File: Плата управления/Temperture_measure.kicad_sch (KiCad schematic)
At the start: 5 parts, among them U8 LMV321

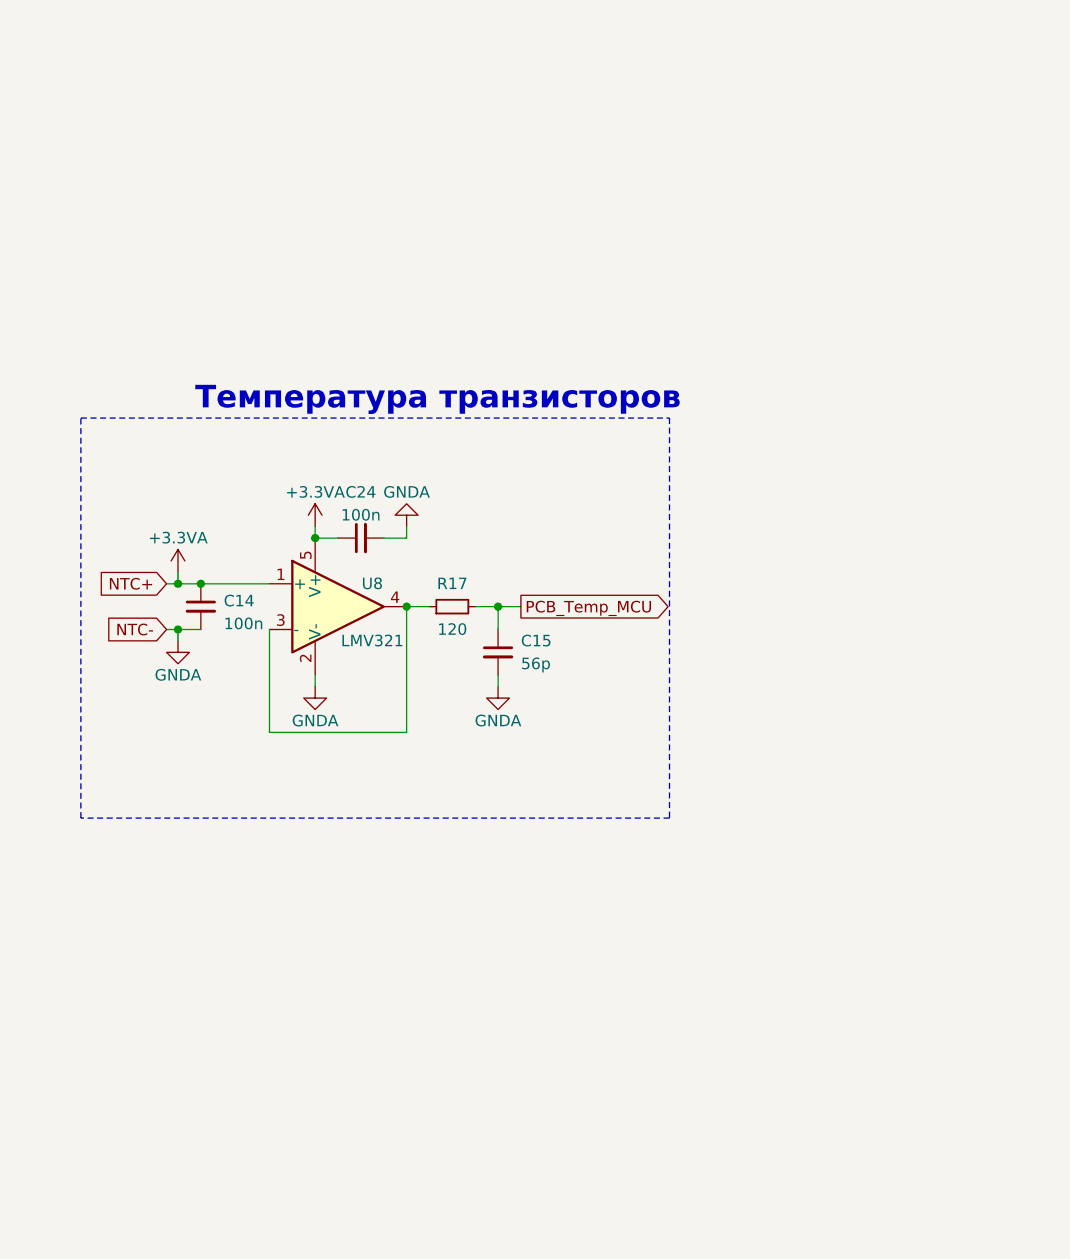
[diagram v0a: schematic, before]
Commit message: Новые драйвера и разъёмы
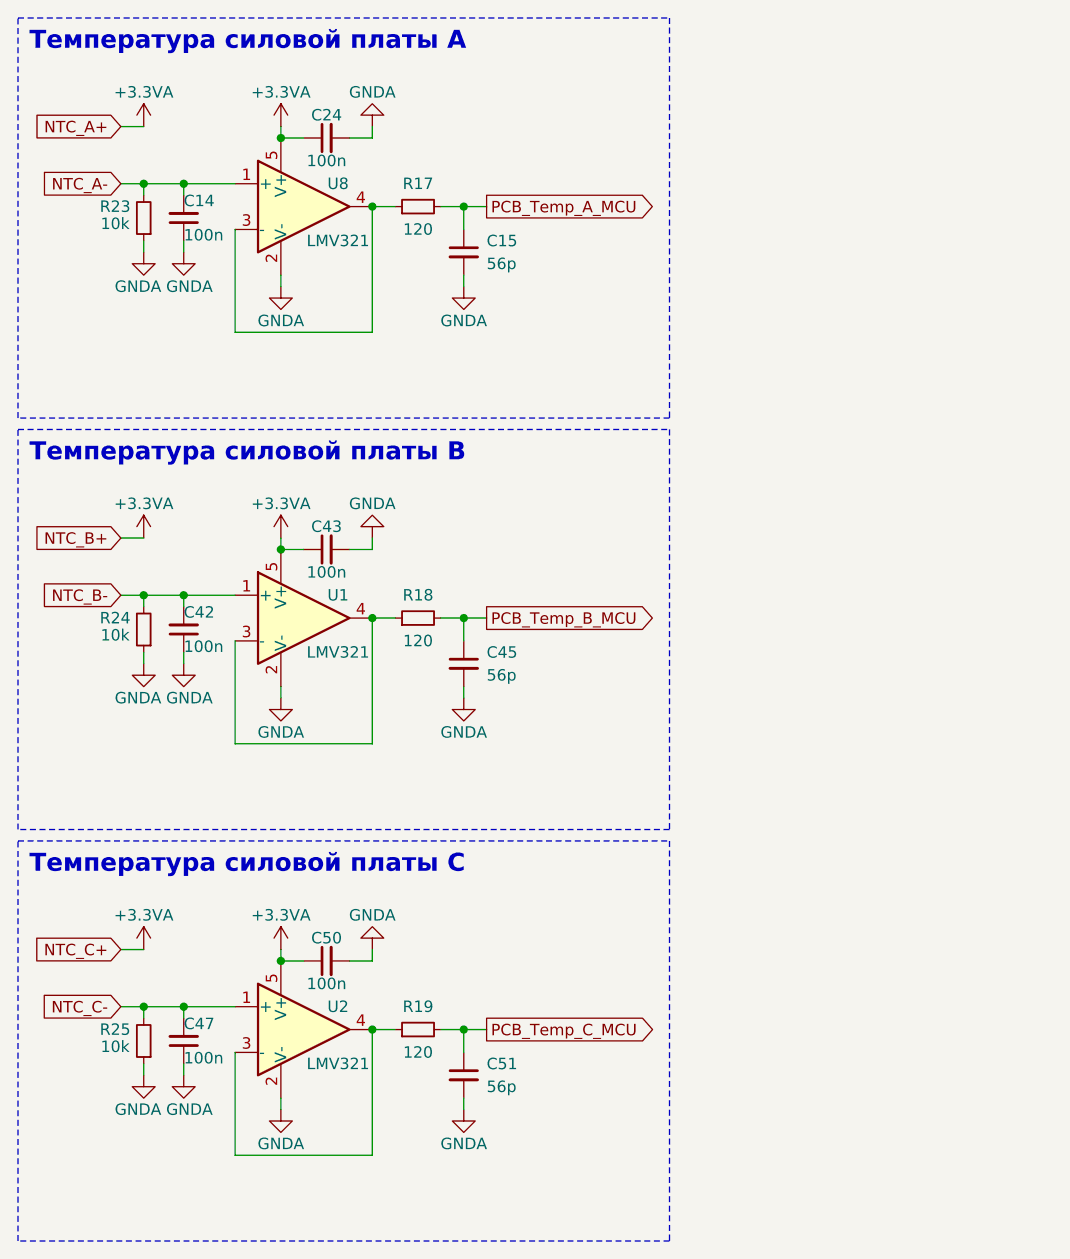
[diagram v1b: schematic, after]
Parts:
- added C42, C43, C47, C50: 100n, Capacitor_SMD:C_0603_1608Metric_Pad1.08x0.95mm_HandSolder, symbol Device:C_Small
- added C45, C51: 56p, Capacitor_SMD:C_0603_1608Metric_Pad1.08x0.95mm_HandSolder, symbol Device:C_Small
- added R18, R19: 120, Resistor_SMD:R_0603_1608Metric_Pad0.98x0.95mm_HandSolder, symbol Device:R_Small
- added R23, R24, R25: 10k, Resistor_SMD:R_0603_1608Metric_Pad0.98x0.95mm_HandSolder, symbol Device:R_Small
- added U1, U2: LMV321, Package_TO_SOT_SMD:SOT-23-5_HandSoldering, symbol Amplifier_Operational:LMV321
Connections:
- net +3.3VA: now also C43.1, C50.1, U1.5 (V+), U2.5 (V+); no longer C14.1, U8.1 (+)
- net GNDA: now also C14.1, C42.1, C43.2, C45.2, C47.1, C50.2, C51.2, R23.1, R24.1, R25.1, U1.2 (V-), U2.2 (V-); no longer C14.2
- net PCB_Temp_MCU renamed PCB_Temp_A_MCU
- new net: R19.1, U2.3 (-), U2.4
- new net: R18.1, U1.3 (-), U1.4
- new net NTC_A-: C14.2, R23.2, U8.1 (+)
- new net NTC_B-: C42.2, R24.2, U1.1 (+)
- new net NTC_C-: C47.2, R25.2, U2.1 (+)
- new net PCB_Temp_B_MCU: C45.1, R18.2
- new net PCB_Temp_C_MCU: C51.1, R19.2
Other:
- note added: "Температура силовой платы A"
- note added: "Температура силовой платы B"
- note added: "Температура силовой платы C"
- note removed: "Температура транзисторов"
- moved on the sheet: C14, C15, C24, R17, U8
